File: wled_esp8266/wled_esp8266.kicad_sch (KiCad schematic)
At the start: 9 parts

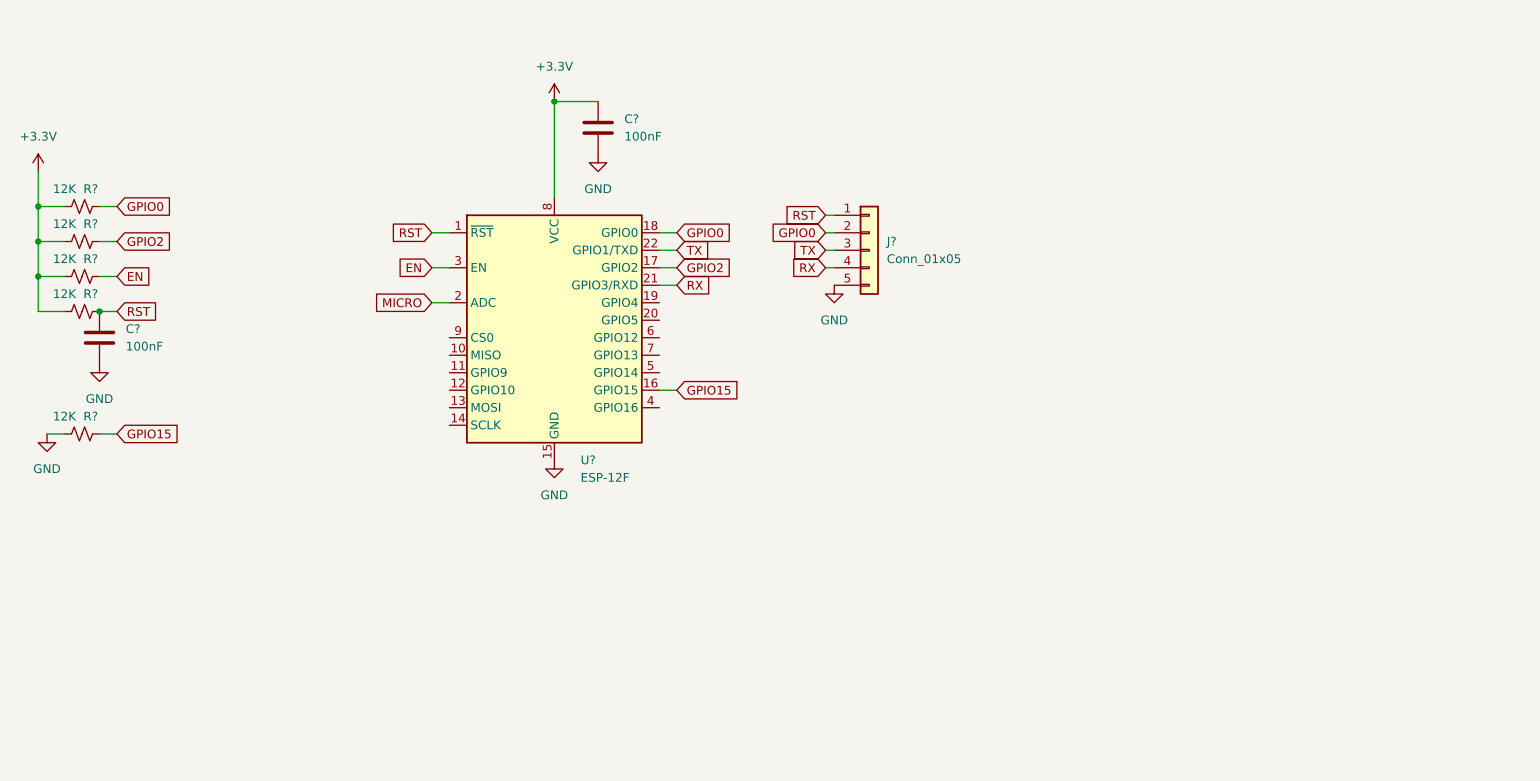
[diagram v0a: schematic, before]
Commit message: update 2
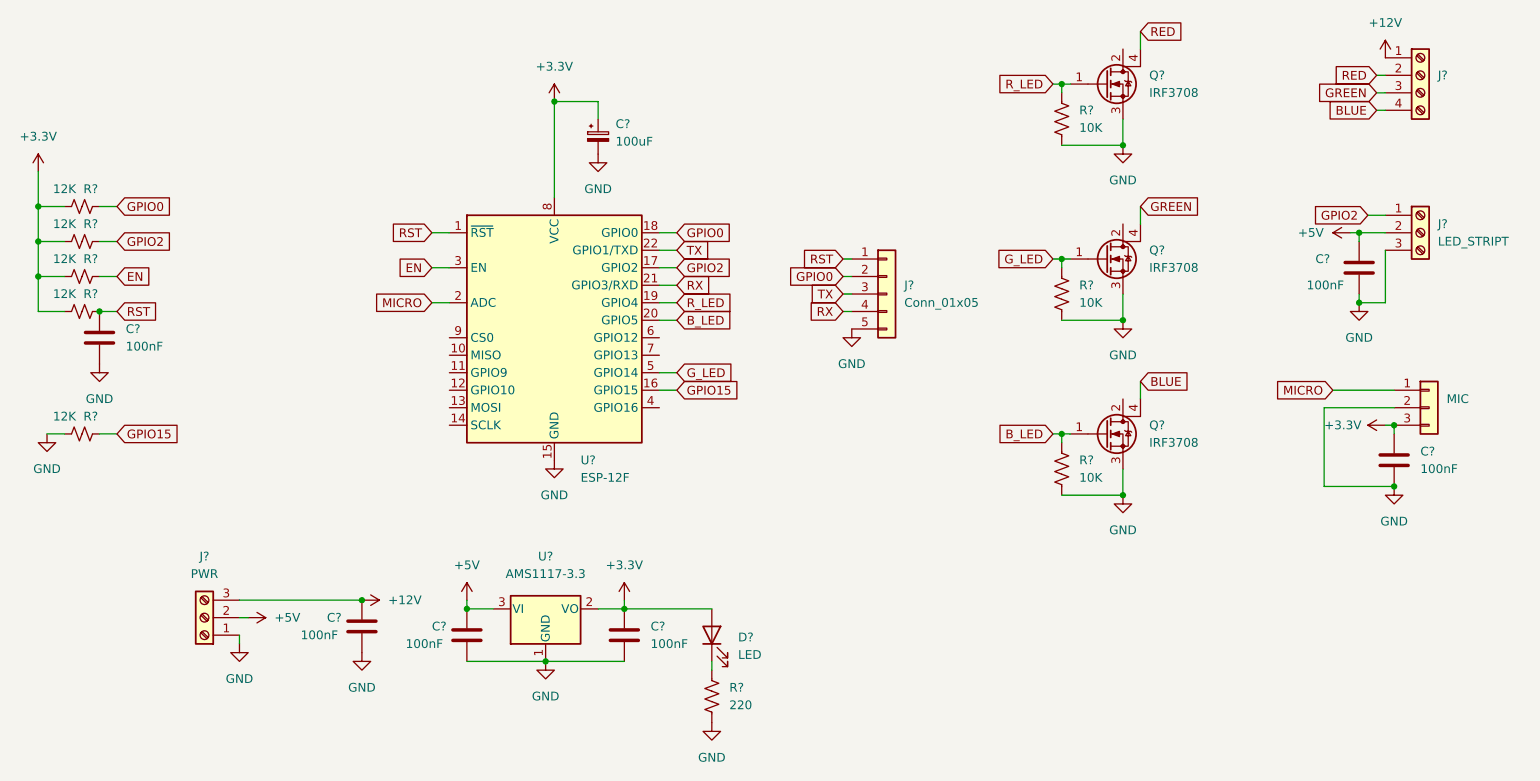
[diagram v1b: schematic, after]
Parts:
- removed C?: 100nF, Capacitor_SMD:C_0805_2012Metric_Pad1.18x1.45mm_HandSolder, symbol Device:C
- added C? (x5): 100nF, Capacitor_SMD:C_0805_2012Metric_Pad1.18x1.45mm_HandSolder, symbol Device:C
- added C?: 100uF, Capacitor_Tantalum_SMD:CP_EIA-3528-12_Kemet-T_Pad1.50x2.35mm_HandSolder, symbol Device:C_Polarized_Small
- added D?: LED, symbol Device:LED
- added J?: LED_STRIPT, symbol Connector:Screw_Terminal_01x03
- added J?: Screw_Terminal_01x04, symbol Connector:Screw_Terminal_01x04
- added J?: PWR, symbol Connector:Screw_Terminal_01x03
- added MIC: Conn_01x03, Connector_PinSocket_2.54mm:PinSocket_1x03_P2.54mm_Vertical, symbol Connector_Generic:Conn_01x03
- added Q? (x3): IRF3708, Package_TO_SOT_SMD:TO-252-3_TabPin4, symbol Device:Q_NMOS_GDSD
- added R? (x3): 10K, Resistor_SMD:R_0805_2012Metric_Pad1.20x1.40mm_HandSolder, symbol Device:R_US
- added R?: 220, Resistor_SMD:R_0805_2012Metric_Pad1.20x1.40mm_HandSolder, symbol Device:R_US
- added U?: AMS1117-3.3, Package_TO_SOT_SMD:SOT-223-3_TabPin2, symbol Regulator_Linear:AMS1117-3.3
- J?: footprint (none) -> Connector_PinSocket_2.54mm:PinSocket_1x05_P2.54mm_Vertical
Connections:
- net +3V3: now also C?.1, C?.1, C?.1, D?.2 (A), MIC.3 (Pin_3), U?.2 (VO)
- net GND: now also C?.2, C?.2, C?.2, C?.2, C?.2, C?.2, J?.1 (Pin_1), J?.3 (Pin_3), MIC.2 (Pin_2), Q?.3 (S), Q?.3 (S), Q?.3 (S), R?.2, R?.2, R?.2, R?.2, U?.1 (GND)
- net GPIO2: now also J?.1 (Pin_1)
- net MICRO: now also MIC.1 (Pin_1)
- net R_LED: now reaches U?.19 (GPIO4)
- net R_LED: now also Q?.1 (G), R?.1
- net B_LED: now reaches U?.20 (GPIO5)
- net B_LED: now also Q?.1 (G), R?.1
- net G_LED: now reaches U?.5 (GPIO14)
- net G_LED: now also Q?.1 (G), R?.1
- new net: D?.1 (K), R?.1
- new net +12V: C?.1, J?.1 (Pin_1), J?.3 (Pin_3)
- new net +5V: C?.1, C?.1, J?.2 (Pin_2), J?.2 (Pin_2), U?.3 (VI)
- new net BLUE: J?.4 (Pin_4), Q?.4 (D)
- new net GREEN: J?.3 (Pin_3), Q?.4 (D)
- new net RED: J?.2 (Pin_2), Q?.4 (D)
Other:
- moved on the sheet: J?
